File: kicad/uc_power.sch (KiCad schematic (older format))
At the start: 29 parts, among them U301 TMS320F28388DZWTS

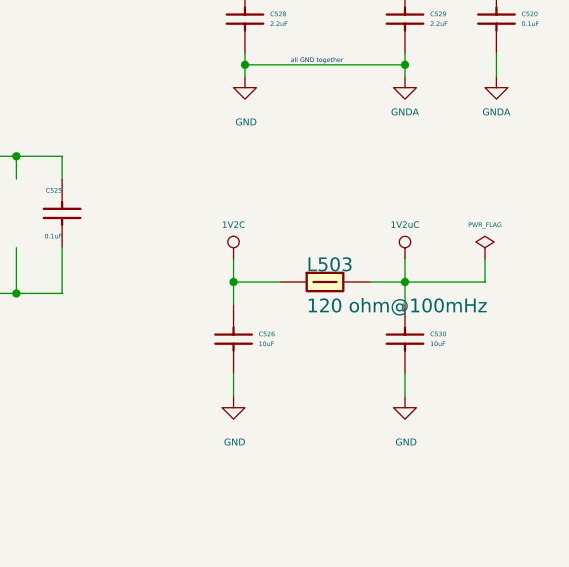
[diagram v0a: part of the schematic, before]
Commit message: stackup
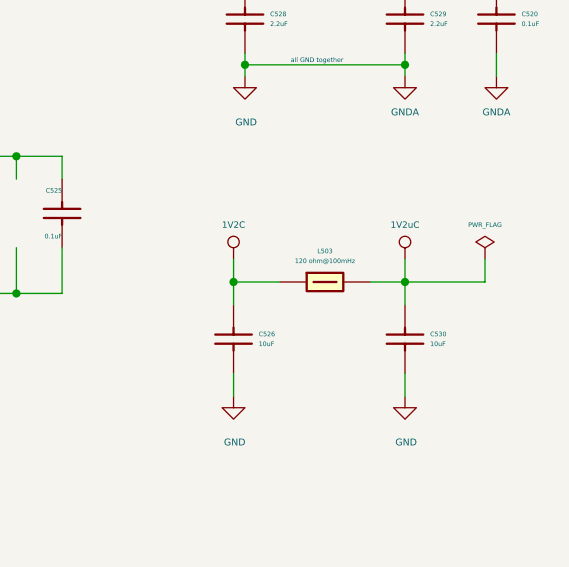
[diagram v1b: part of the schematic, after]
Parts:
- C501, C502, C503, C504, C505, C506, C507, C511, C512, C514, C515, C516, C517, C518, C519, C520, C521, C523, C524, C525: price@10 (none) -> 0.05800
- C526, C530: price@10 (none) -> 0.15400
- C528, C529, C531: digikey 490-12287-2-ND -> 490-12287-1-ND; price@10 (none) -> 0.35500
